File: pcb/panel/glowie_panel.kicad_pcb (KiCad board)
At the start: 2 copper layers, 12 x 12 mm, 10 parts, among them J1 Conn_01x04, J3 Conn_01x01, J4 Conn_01x01, J5 USB_C_Receptacle_USB2.0_16P, J6 Conn_01x01, SW1 SW_Push, U1 USBLC6-2SC6

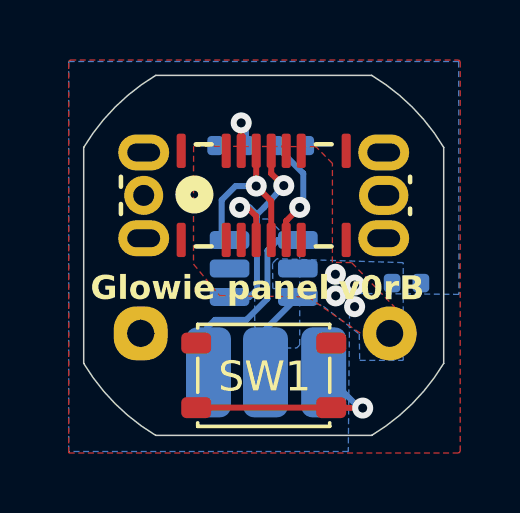
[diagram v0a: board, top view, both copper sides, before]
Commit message: Panel routing improvements
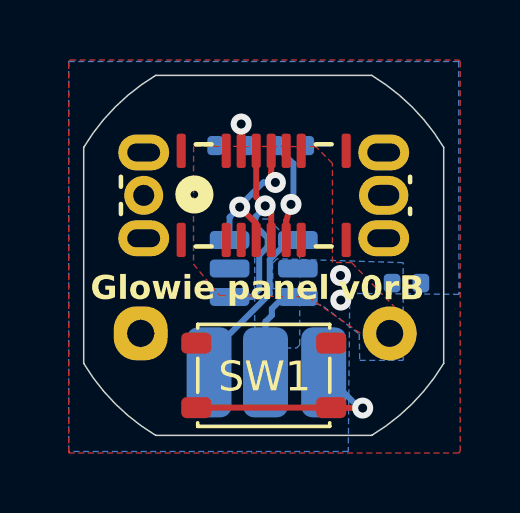
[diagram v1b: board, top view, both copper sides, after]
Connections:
- J1 pad 1: /USB_D- -> /USB_D+
- J1 pad 2: /USB_D+ -> /USB_D-
- U1 pad 1: Net-(J5-D--PadA7) -> Net-(J5-D+-PadA6)
- U1 pad 3: Net-(J5-D+-PadA6) -> Net-(J5-D--PadA7)
- U1 pad 4: /USB_D+ -> /USB_D-
- U1 pad 6: /USB_D- -> /USB_D+
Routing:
- net /USB_D+: track 6.66 -> 3.24 mm
- net Net-(J5-D--PadA7): track 8.30 -> 5.16 mm
- net /USB_D-: track 3.30 -> 5.80 mm
- net Net-(J5-D+-PadA6): track 6.10 -> 7.48 mm
- net /USB_VBUS: vias 4 -> 2
